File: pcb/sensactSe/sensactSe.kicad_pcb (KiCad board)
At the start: 2 copper layers, 27.4 x 33.5 mm, 25 parts, among them P1 Input, P2 CONN_01X07, P3 CONN_01X07, P4 CONN_01X01, P5 OUTPUT, U1 TLV70033DDC, U2 STM32F030F4, U3 NUD3124DMT1G, U4 SRV05, U5 DS18B20, U6 DS2413

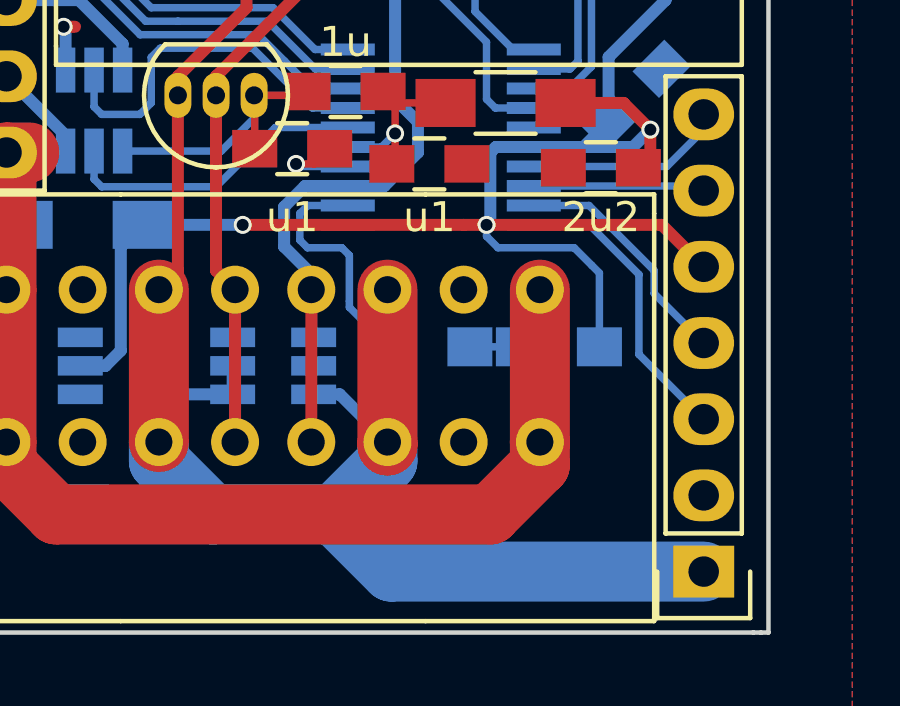
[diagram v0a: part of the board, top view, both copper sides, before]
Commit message: sensactSE Changes
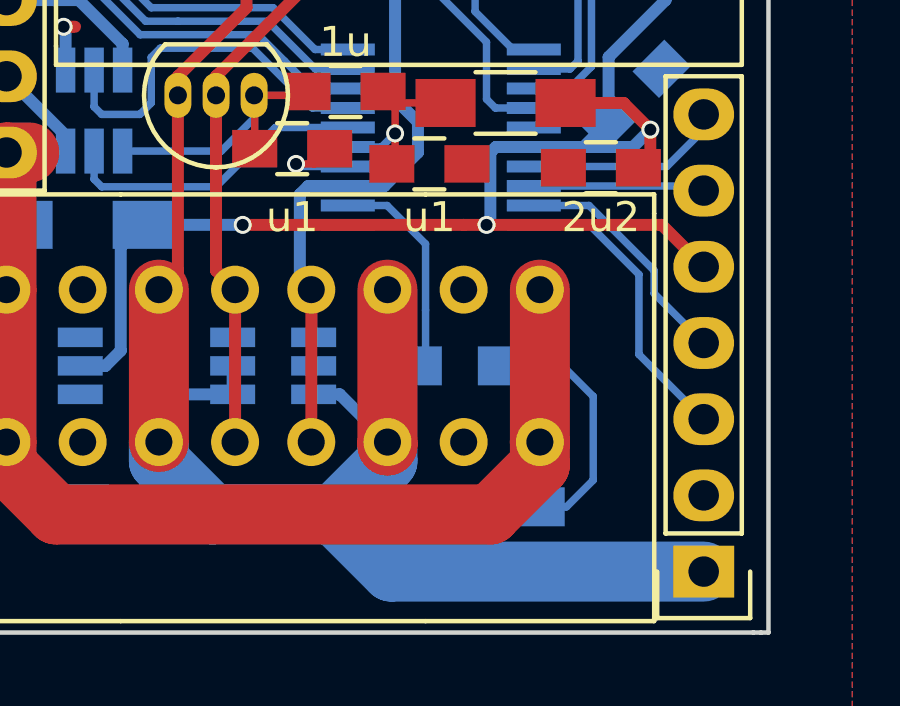
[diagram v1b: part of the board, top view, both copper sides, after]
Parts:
- moved R4 5.66 mm to (117.9, 100.2), turned to 0 degrees
- moved D1 1.20 mm to (116.5, 95.5), turned to 180 degrees
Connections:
- R4 pad 1: +3V3 -> GND
- R4 pad 2: Net-(D1-Pad2) -> Net-(D1-Pad1)
- U2 pad 2: Net-(D1-Pad1) -> Net-(D1-Pad2)
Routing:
- net +3V3: track 68.0 -> 60.9 mm
- net Net-(D1-Pad2): track 1.62 -> 7.27 mm
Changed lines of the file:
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@@
     (thickness 1.6)
     (drawings 13)
-    (tracks 244)
+    (tracks 237)
     (zones 0)
     (modules 25)
@@
   (layers
     (0 F.Cu signal)
-    (31 B.Cu signal hide)
+    (31 B.Cu signal)
     (32 B.Adhes user)
     (33 F.Adhes user hide)
@@
   )
   (setup
-    (last_trace_width 0.4)
+    (last_trace_width 0.25)
     (user_trace_width 0.25)
     (user_trace_width 0.4)
@@
       (net 2 GND))
     (pad 2 smd rect (at -3.1 2.275) (size 1.8 0.4) (layers B.Cu B.Paste B.Mask)
-      (net 24 "Net-(D1-Pad1)"))
+      (net 25 "Net-(D1-Pad2)"))
     (pad 3 smd rect (at -3.1 1.625) (size 1.8 0.4) (layers B.Cu B.Paste B.Mask)
       (net 21 /1Wr))
@@
   )
   (module Resistors_SMD:R_0805_HandSoldering (layer B.Cu)
-    (at 115.443 94.869)
+    (at 116.459 95.504 180)
     (descr "Resistor SMD 0805, hand soldering")
     (tags "resistor 0805")
     (attr smd)
-    (fp_text reference D1 (at 0 2.1) (layer B.SilkS)
-      (effects (font (size 1 1) (thickness 0.15)) (justify mirror))
-    )
-    (fp_text value LED (at 0 -2.1) (layer B.Fab)
+    (fp_text reference D1 (at 0 2.1 180) (layer B.SilkS)
+      (effects (font (size 1 1) (thickness 0.15)) (justify mirror))
+    )
+    (fp_text value LED (at 0 -2.1 180) (layer B.Fab) hide
+      (effects (font (size 1 1) (thickness 0.15)) (justify mirror))
+    )
+    (fp_line (start -2.4 1) (end 2.4 1) (layer B.CrtYd) (width 0.05))
+    (fp_line (start -2.4 -1) (end 2.4 -1) (layer B.CrtYd) (width 0.05))
+    (fp_line (start -2.4 1) (end -2.4 -1) (layer B.CrtYd) (width 0.05))
+    (fp_line (start 2.4 1) (end 2.4 -1) (layer B.CrtYd) (width 0.05))
+    (fp_line (start 0.6 -0.875) (end -0.6 -0.875) (layer B.SilkS) (width 0.15))
+    (fp_line (start -0.6 0.875) (end 0.6 0.875) (layer B.SilkS) (width 0.15))
+    (pad 1 smd rect (at -1.35 0 180) (size 1.5 1.3) (layers B.Cu B.Paste B.Mask)
+      (net 24 "Net-(D1-Pad1)"))
+    (pad 2 smd rect (at 1.35 0 180) (size 1.5 1.3) (layers B.Cu B.Paste B.Mask)
+      (net 25 "Net-(D1-Pad2)"))
+    (model Resistors_SMD.3dshapes/R_0805_HandSoldering.wrl
+      (at (xyz 0 0 0))
+      (scale (xyz 1 1 1))
+      (rotate (xyz 0 0 0))
+    )
+  )
+  (module Resistors_SMD:R_0805_HandSoldering (layer B.Cu)
+    (at 117.856 100.203)
+    (descr "Resistor SMD 0805, hand soldering")
+    (tags "resistor 0805")
+    (attr smd)
+    (fp_text reference R4 (at 0 2.1) (layer B.SilkS)
+      (effects (font (size 1 1) (thickness 0.15)) (justify mirror))
+    )
+    (fp_text value k1 (at 1.397 -5.334) (layer B.SilkS)
       (effects (font (size 1 1) (thickness 0.15)) (justify mirror))
     )
@@
     (fp_line (start -0.6 0.875) (end 0.6 0.875) (layer B.SilkS) (width 0.15))
     (pad 1 smd rect (at -1.35 0) (size 1.5 1.3) (layers B.Cu B.Paste B.Mask)
+      (net 2 GND))
+    (pad 2 smd rect (at 1.35 0) (size 1.5 1.3) (layers B.Cu B.Paste B.Mask)
       (net 24 "Net-(D1-Pad1)"))
-    (pad 2 smd rect (at 1.35 0) (size 1.5 1.3) (layers B.Cu B.Paste B.Mask)
-      (net 25 "Net-(D1-Pad2)"))
-    (model Resistors_SMD.3dshapes/R_0805_HandSoldering.wrl
-      (at (xyz 0 0 0))
-      (scale (xyz 1 1 1))
-      (rotate (xyz 0 0 0))
-    )
-  )
-  (module Resistors_SMD:R_0805_HandSoldering (layer B.Cu)
-    (at 119.761 94.869 180)
-    (descr "Resistor SMD 0805, hand soldering")
-    (tags "resistor 0805")
-    (attr smd)
-    (fp_text reference R4 (at 0 2.1 180) (layer B.SilkS)
-      (effects (font (size 1 1) (thickness 0.15)) (justify mirror))
-    )
-    (fp_text value k1 (at 0 -2.1 180) (layer B.Fab)
-      (effects (font (size 1 1) (thickness 0.15)) (justify mirror))
-    )
-    (fp_line (start -2.4 1) (end 2.4 1) (layer B.CrtYd) (width 0.05))
-    (fp_line (start -2.4 -1) (end 2.4 -1) (layer B.CrtYd) (width 0.05))
-    (fp_line (start -2.4 1) (end -2.4 -1) (layer B.CrtYd) (width 0.05))
-    (fp_line (start 2.4 1) (end 2.4 -1) (layer B.CrtYd) (width 0.05))
-    (fp_line (start 0.6 -0.875) (end -0.6 -0.875) (layer B.SilkS) (width 0.15))
-    (fp_line (start -0.6 0.875) (end 0.6 0.875) (layer B.SilkS) (width 0.15))
-    (pad 1 smd rect (at -1.35 0 180) (size 1.5 1.3) (layers B.Cu B.Paste B.Mask)
-      (net 3 +3V3))
-    (pad 2 smd rect (at 1.35 0 180) (size 1.5 1.3) (layers B.Cu B.Paste B.Mask)
-      (net 25 "Net-(D1-Pad2)"))
     (model Resistors_SMD.3dshapes/R_0805_HandSoldering.wrl
       (at (xyz 0 0 0))
@@
   (via (at 103.251 84.201) (size 0.6) (drill 0.4) (layers F.Cu B.Cu) (net 2))
   (segment (start 103.317 84.267) (end 103.251 84.201) (width 0.4) (layer B.Cu) (net 2))
-  (segment (start 120.857 92.155) (end 121.111 92.409) (width 0.25) (layer B.Cu) (net 3))
-  (segment (start 120.269 91.567) (end 120.857 92.155) (width 0.25) (layer B.Cu) (net 3))
-  (segment (start 117.348 90.805) (end 117.348 91.186) (width 0.25) (layer B.Cu) (net 3))
-  (segment (start 117.348 91.186) (end 117.729 91.567) (width 0.25) (layer B.Cu) (net 3))
-  (segment (start 117.729 91.567) (end 120.269 91.567) (width 0.25) (layer B.Cu) (net 3))
-  (segment (start 121.111 92.409) (end 121.111 94.869) (width 0.25) (layer B.Cu) (net 3))
   (segment (start 118.924 88.209) (end 117.658 88.209) (width 0.4) (layer B.Cu) (net 3))
   (segment (start 117.348 90.805) (end 117.221 90.805) (width 0.4) (layer F.Cu) (net 3))
@@
   (segment (start 112.724 88.209) (end 113.848 88.209) (width 0.25) (layer B.Cu) (net 20))
   (segment (start 113.848 88.209) (end 114.3 87.757) (width 0.25) (layer B.Cu) (net 20))
+  (segment (start 112.724 89.509) (end 111.405 89.509) (width 0.4) (layer B.Cu) (net 21))
+  (segment (start 111.125 89.789) (end 111.125 92.583) (width 0.4) (layer B.Cu) (net 21))
+  (segment (start 111.405 89.509) (end 111.125 89.789) (width 0.4) (layer B.Cu) (net 21))
+  (segment (start 111.125 92.583) (end 111.506 92.964) (width 0.4) (layer B.Cu) (net 21))
   (segment (start 112.724 89.509) (end 113.945 89.509) (width 0.4) (layer B.Cu) (net 21))
   (segment (start 114.3 86.614) (end 114.3 82.423) (width 0.4) (layer B.Cu) (net 21))
@@
   (segment (start 114.427 77.216) (end 114.427 74.977) (width 0.4) (layer B.Cu) (net 21))
   (segment (start 114.427 74.977) (end 114.38 74.93) (width 0.4) (layer B.Cu) (net 21))
-  (segment (start 111.506 92.964) (end 111.506 92.436464) (width 0.4) (layer B.Cu) (net 21))
-  (segment (start 111.506 92.436464) (end 110.599998 91.530462) (width 0.4) (layer B.Cu) (net 21))
-  (segment (start 111.297536 89.509) (end 112.724 89.509) (width 0.4) (layer B.Cu) (net 21))
-  (segment (start 110.599998 90.206538) (end 111.297536 89.509) (width 0.4) (layer B.Cu) (net 21))
-  (segment (start 110.599998 91.530462) (end 110.599998 90.206538) (width 0.4) (layer B.Cu) (net 21))
   (segment (start 114.173 82.55) (end 114.427 82.296) (width 0.4) (layer B.Cu) (net 21))
   (segment (start 114.427 77.216) (end 114.427 82.296) (width 0.4) (layer F.Cu) (net 21))
@@
   (segment (start 118.924 86.909) (end 117.643 86.909) (width 0.25) (layer B.Cu) (net 23))
   (segment (start 109.289002 80.968002) (end 108.077 79.756) (width 0.25) (layer B.Cu) (net 23))
-  (segment (start 112.776 91.821) (end 112.776 93.345) (width 0.25) (layer B.Cu) (net 24))
-  (segment (start 111.39 90.159) (end 111.125 90.424) (width 0.25) (layer B.Cu) (net 24))
-  (segment (start 111.125 90.424) (end 111.125 91.313) (width 0.25) (layer B.Cu) (net 24))
-  (segment (start 111.125 91.313) (end 111.379 91.567) (width 0.25) (layer B.Cu) (net 24))
-  (segment (start 111.379 91.567) (end 112.522 91.567) (width 0.25) (layer B.Cu) (net 24))
-  (segment (start 112.522 91.567) (end 112.776 91.821) (width 0.25) (layer B.Cu) (net 24))
-  (segment (start 112.724 90.159) (end 111.39 90.159) (width 0.25) (layer B.Cu) (net 24))
-  (segment (start 112.776 93.552) (end 114.093 94.869) (width 0.25) (layer B.Cu) (net 24))
-  (segment (start 112.776 93.345) (end 112.776 93.552) (width 0.25) (layer B.Cu) (net 24))
-  (segment (start 118.411 94.869) (end 116.793 94.869) (width 0.25) (layer B.Cu) (net 25))
+  (segment (start 117.809 95.504) (end 119.888 95.504) (width 0.25) (layer B.Cu) (net 24))
+  (segment (start 120.015 100.203) (end 119.206 100.203) (width 0.25) (layer B.Cu) (net 24))
+  (segment (start 120.904 99.314) (end 120.015 100.203) (width 0.25) (layer B.Cu) (net 24))
+  (segment (start 120.904 96.52) (end 120.904 99.314) (width 0.25) (layer B.Cu) (net 24))
+  (segment (start 119.888 95.504) (end 120.904 96.52) (width 0.25) (layer B.Cu) (net 24))
+  (segment (start 115.316 95.297) (end 115.316 93.646) (width 0.25) (layer B.Cu) (net 25))
+  (segment (start 114.035 90.159) (end 115.316 91.44) (width 0.25) (layer B.Cu) (net 25))
+  (segment (start 115.316 91.44) (end 115.316 93.646) (width 0.25) (layer B.Cu) (net 25))
+  (segment (start 114.035 90.159) (end 112.724 90.159) (width 0.25) (layer B.Cu) (net 25))
+  (segment (start 115.316 95.297) (end 115.109 95.504) (width 0.25) (layer B.Cu) (net 25))
   (zone (net 2) (net_name GND) (layer F.Cu) (hatch edge 0.508)
     (connect_pads (clearance 0.3))
